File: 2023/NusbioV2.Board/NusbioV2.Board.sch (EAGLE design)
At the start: 27 parts

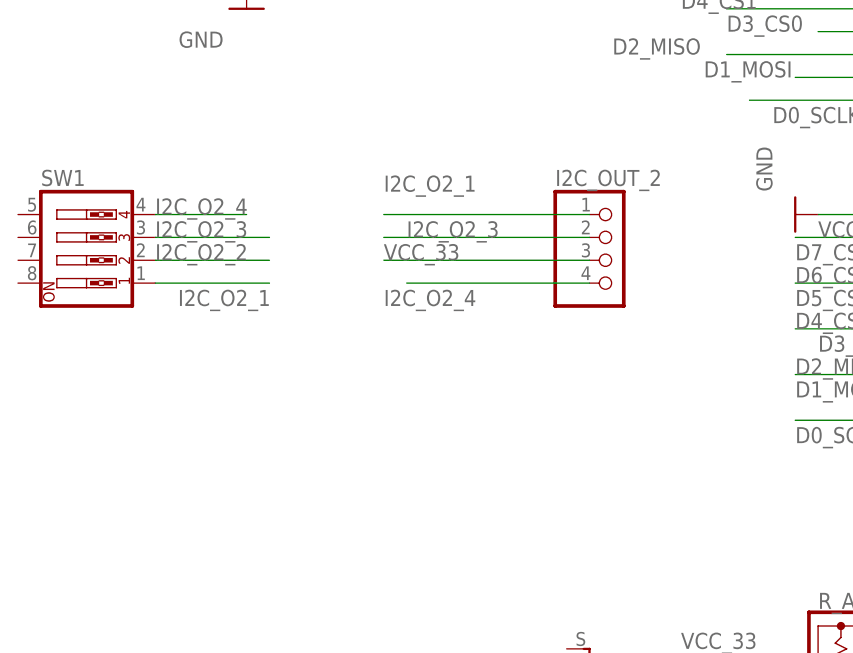
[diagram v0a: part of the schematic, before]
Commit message: Nsubio /2 v2 update
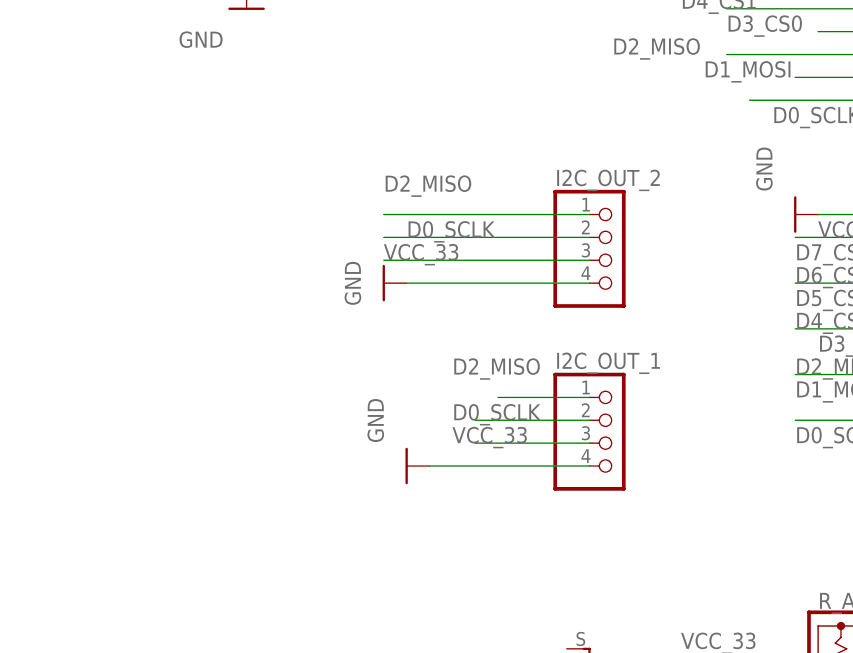
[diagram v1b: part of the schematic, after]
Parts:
- removed SW1: (no value), special:SW_DIP-4
- added I2C_OUT_1: (no value), pinhead:PINHD-1X4
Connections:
- removed net I2C_O2_1: I2C_OUT_2.1, SW1.1
- removed net I2C_O2_2: SW1.2
- removed net I2C_O2_3: I2C_OUT_2.2, SW1.3
- removed net I2C_O2_4: I2C_OUT_2.4, SW1.4
- net D0_SCLK: now also I2C_OUT_1.2, I2C_OUT_2.2
- net D2_MISO: now also I2C_OUT_1.1, I2C_OUT_2.1
- net GND: now also I2C_OUT_1.4, I2C_OUT_2.4
- net VCC_33: now also I2C_OUT_1.3
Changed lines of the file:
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@@
 <part name="JP_5V" library="pinhead" library_urn="urn:adsk.eagle:library:325" deviceset="PINHD-1X2" device="" package3d_urn="urn:adsk.eagle:package:22435/2"/>
 <part name="GND8" library="supply1" deviceset="GND" device=""/>
+<part name="I2C_OUT_1" library="pinhead" library_urn="urn:adsk.eagle:library:325" deviceset="PINHD-1X4" device="" package3d_urn="urn:adsk.eagle:package:22407/2"/>
+<part name="GND9" library="supply1" deviceset="GND" device=""/>
 <part name="I2C_PULL_UP_MODE" library="adafruit" deviceset="EG1218" device="S"/>
 <part name="R_PULL_UP_SCL_4K" library="adafruit" deviceset="R-US_" device="R1206"/>
 <part name="R_PULL_UP_SDA_4K" library="adafruit" deviceset="R-US_" device="R1206"/>
 <part name="I2C_OUT_2" library="pinhead" library_urn="urn:adsk.eagle:library:325" deviceset="PINHD-1X4" device="" package3d_urn="urn:adsk.eagle:package:22407/2"/>
+<part name="GND10" library="supply1" deviceset="GND" device=""/>
 <part name="I2C_DTA_CONN" library="adafruit" deviceset="EG1218" device="S"/>
 <part name="H1" library="holes" library_urn="urn:adsk.eagle:library:237" deviceset="MOUNT-PAD-ROUND" device="3.3" package3d_urn="urn:adsk.eagle:package:14283/1"/>
@@
 <part name="H3" library="holes" library_urn="urn:adsk.eagle:library:237" deviceset="MOUNT-PAD-ROUND" device="3.3" package3d_urn="urn:adsk.eagle:package:14283/1"/>
 <part name="H4" library="holes" library_urn="urn:adsk.eagle:library:237" deviceset="MOUNT-PAD-ROUND" device="3.3" package3d_urn="urn:adsk.eagle:package:14283/1"/>
-<part name="SW1" library="special" library_urn="urn:adsk.eagle:library:367" deviceset="SW_DIP-4" device="" package3d_urn="urn:adsk.eagle:package:26655/2"/>
 </parts>
 <sheets>
@@
 <attribute name="VALUE" x="-17.78" y="160.02" size="1.778" layer="96" rot="R90"/>
 </instance>
+<instance part="I2C_OUT_1" gate="A" x="-119.38" y="99.06" smashed="yes">
+<attribute name="NAME" x="-125.73" y="107.315" size="1.778" layer="95"/>
+<attribute name="VALUE" x="-125.73" y="91.44" size="1.778" layer="96"/>
+</instance>
+<instance part="GND9" gate="1" x="-142.24" y="96.52" smashed="yes" rot="R270">
+<attribute name="VALUE" x="-144.78" y="99.06" size="1.778" layer="96" rot="R90"/>
+</instance>
 <instance part="I2C_PULL_UP_MODE" gate="1" x="-119.38" y="71.12" smashed="yes" rot="R90">
 <attribute name="NAME" x="-104.775" y="67.31" size="1.778" layer="95" rot="R180"/>
@@
 <attribute name="VALUE" x="-125.73" y="111.76" size="1.778" layer="96"/>
 </instance>
+<instance part="GND10" gate="1" x="-144.78" y="116.84" smashed="yes" rot="R270">
+<attribute name="VALUE" x="-147.32" y="114.3" size="1.778" layer="96" rot="R90"/>
+</instance>
 <instance part="I2C_DTA_CONN" gate="1" x="-137.16" y="40.64" smashed="yes" rot="R90">
 <attribute name="NAME" x="-122.555" y="36.83" size="1.778" layer="95" rot="R180"/>
@@
 <attribute name="NAME" x="-83.566" y="180.9242" size="1.778" layer="95"/>
 <attribute name="VALUE" x="-83.566" y="177.8762" size="1.778" layer="96"/>
-</instance>
-<instance part="SW1" gate="A" x="-177.8" y="121.92" smashed="yes">
-<attribute name="NAME" x="-182.88" y="127.635" size="1.778" layer="95"/>
-<attribute name="VALUE" x="-182.88" y="111.76" size="1.778" layer="96"/>
 </instance>
 </instances>
@@
 <pinref part="GND8" gate="1" pin="GND"/>
 <wire x1="2.54" y1="157.48" x2="-12.7" y2="157.48" width="0.1524" layer="91"/>
+</segment>
+<segment>
+<pinref part="I2C_OUT_1" gate="A" pin="4"/>
+<pinref part="GND9" gate="1" pin="GND"/>
+<wire x1="-121.92" y1="96.52" x2="-139.7" y2="96.52" width="0.1524" layer="91"/>
+</segment>
+<segment>
+<pinref part="I2C_OUT_2" gate="A" pin="4"/>
+<pinref part="GND10" gate="1" pin="GND"/>
+<wire x1="-121.92" y1="116.84" x2="-142.24" y2="116.84" width="0.1524" layer="91"/>
 </segment>
 <segment>
@@
 </segment>
 <segment>
+<pinref part="I2C_OUT_1" gate="A" pin="3"/>
+<wire x1="-121.92" y1="99.06" x2="-134.62" y2="99.06" width="0.1524" layer="91"/>
+<label x="-137.16" y="99.06" size="1.778" layer="95"/>
+</segment>
+<segment>
 <pinref part="I2C_PULL_UP_MODE" gate="1" pin="P"/>
 <wire x1="-114.3" y1="73.66" x2="-104.14" y2="73.66" width="0.1524" layer="91"/>
@@
 <label x="-162.56" y="68.58" size="1.778" layer="95"/>
 </segment>
+<segment>
+<pinref part="I2C_OUT_2" gate="A" pin="2"/>
+<wire x1="-121.92" y1="121.92" x2="-144.78" y2="121.92" width="0.1524" layer="91"/>
+<label x="-142.24" y="121.92" size="1.778" layer="95"/>
+</segment>
+<segment>
+<pinref part="I2C_OUT_1" gate="A" pin="2"/>
+<wire x1="-121.92" y1="101.6" x2="-134.62" y2="101.6" width="0.1524" layer="91"/>
+<label x="-137.16" y="101.6" size="1.778" layer="95"/>
+</segment>
 </net>
 <net name="D1_MOSI" class="0">
@@
 <wire x1="-142.24" y1="40.64" x2="-160.02" y2="40.64" width="0.1524" layer="91"/>
 <label x="-162.56" y="43.18" size="1.778" layer="95"/>
+</segment>
+<segment>
+<pinref part="I2C_OUT_2" gate="A" pin="1"/>
+<wire x1="-121.92" y1="124.46" x2="-144.78" y2="124.46" width="0.1524" layer="91"/>
+<label x="-144.78" y="127" size="1.778" layer="95"/>
+</segment>
+<segment>
+<pinref part="I2C_OUT_1" gate="A" pin="1"/>
+<wire x1="-121.92" y1="104.14" x2="-132.08" y2="104.14" width="0.1524" layer="91"/>
+<label x="-137.16" y="106.68" size="1.778" layer="95"/>
 </segment>
 </net>
@@
 </segment>
 </net>
-<net name="I2C_O2_4" class="0">
-<segment>
-<pinref part="I2C_OUT_2" gate="A" pin="4"/>
-<wire x1="-121.92" y1="116.84" x2="-142.24" y2="116.84" width="0.1524" layer="91"/>
-<label x="-144.78" y="114.3" size="1.778" layer="95"/>
-</segment>
-<segment>
-<pinref part="SW1" gate="A" pin="4"/>
-<wire x1="-170.18" y1="124.46" x2="-160.02" y2="124.46" width="0.1524" layer="91"/>
-<label x="-170.18" y="124.46" size="1.778" layer="95"/>
-</segment>
-</net>
-<net name="I2C_O2_1" class="0">
-<segment>
-<pinref part="I2C_OUT_2" gate="A" pin="1"/>
-<wire x1="-121.92" y1="124.46" x2="-144.78" y2="124.46" width="0.1524" layer="91"/>
-<label x="-144.78" y="127" size="1.778" layer="95"/>
-</segment>
-<segment>
-<pinref part="SW1" gate="A" pin="1"/>
-<wire x1="-170.18" y1="116.84" x2="-157.48" y2="116.84" width="0.1524" layer="91"/>
-<label x="-167.64" y="114.3" size="1.778" layer="95"/>
-</segment>
-</net>
-<net name="I2C_O2_3" class="0">
-<segment>
-<pinref part="I2C_OUT_2" gate="A" pin="2"/>
-<wire x1="-121.92" y1="121.92" x2="-144.78" y2="121.92" width="0.1524" layer="91"/>
-<label x="-142.24" y="121.92" size="1.778" layer="95"/>
-</segment>
-<segment>
-<pinref part="SW1" gate="A" pin="3"/>
-<wire x1="-170.18" y1="121.92" x2="-157.48" y2="121.92" width="0.1524" layer="91"/>
-<label x="-170.18" y="121.92" size="1.778" layer="95"/>
-</segment>
-</net>
-<net name="I2C_O2_2" class="0">
-<segment>
-<pinref part="SW1" gate="A" pin="2"/>
-<wire x1="-170.18" y1="119.38" x2="-157.48" y2="119.38" width="0.1524" layer="91"/>
-<label x="-170.18" y="119.38" size="1.778" layer="95"/>
-</segment>
-</net>
